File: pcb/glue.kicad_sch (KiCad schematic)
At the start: 63 parts, among them SW1 Opts, SW2 Reset Vector, SW3 NMI, SW4 RESET, U10 GAL16V8, U12 MCP100-475D, U2 74LS573, U3 74LS573, U4 74LS245, U5 74LS245, U6 74AHC273, U7 74LS240, U8 74LS240, U9 74LS259

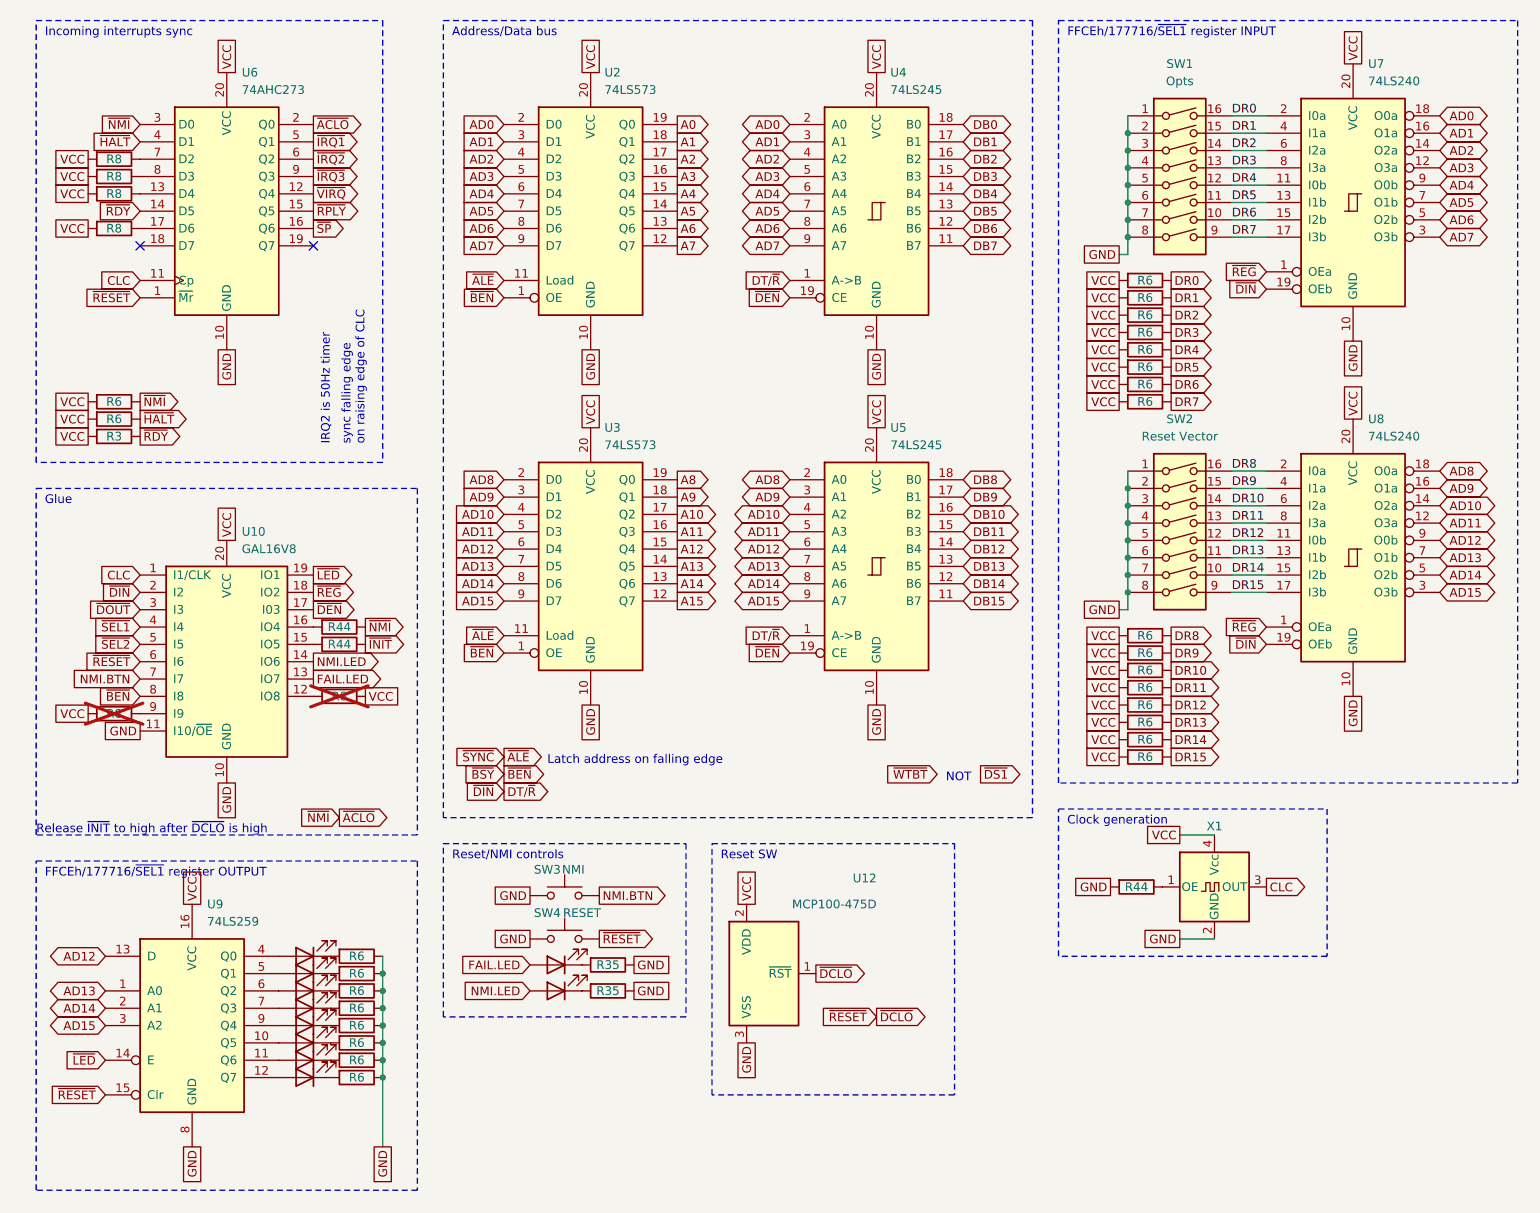
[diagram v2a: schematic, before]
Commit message: full? schematics
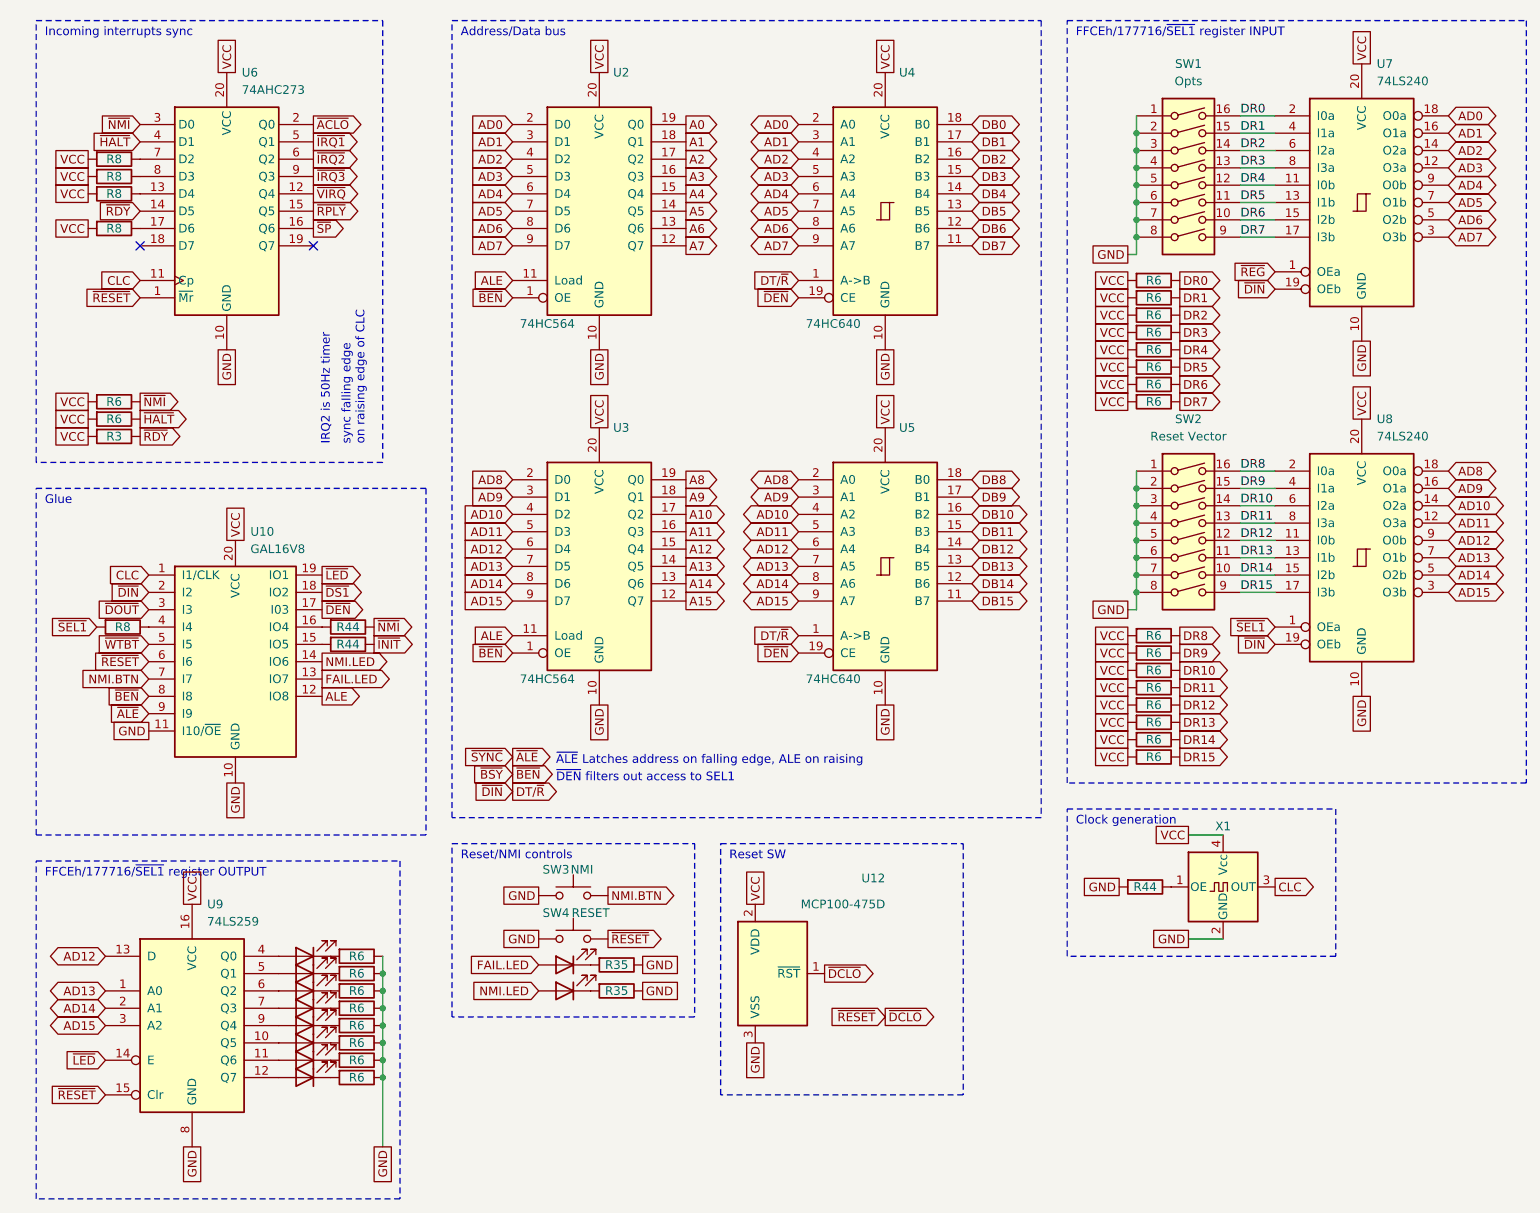
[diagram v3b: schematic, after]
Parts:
- removed R8 (x2): 0R, Resistor_SMD:R_0603_1608Metric_Pad0.98x0.95mm_HandSolder, symbol Device:R
- added R8: 0R, Resistor_SMD:R_0603_1608Metric_Pad0.98x0.95mm_HandSolder, symbol Device:R
- SW3, SW4: footprint (none) -> Button_Switch_THT:SW_SPST_Omron_B3F-315x_Angled
- U12: footprint (none) -> Package_TO_SOT_SMD:SOT-23-3
- U2, U3: value 74LS573 -> 74HC564; symbol 74xx:74LS573 -> 74xx_EXTRA:74LS564; Manufacturer_Part_Number 74VHCT573AFT -> (none); RS Part Number 171-3540 -> (none)
- U4, U5: value 74LS245 -> 74HC640; symbol 74xx:74LS245 -> 74xx_EXTRA:74LS640; Manufacturer_Name Texas Instruments -> (none); Manufacturer_Part_Number MC74HCT245ADWG -> (none); Mouser Part Number 863-MC74HCT245ADWG -> (none)
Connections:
- net ~{SEL2} is gone; now on net ~{WTBT}: U10.5 (I5)
- net ~{ACLO}: no longer R44.1, R6.1, U6.3 (D0)
- net ~{ALE}: now also U10.9 (I9); no longer U2.11 (Load), U3.11 (Load)
- net ~{DS1}: now also U10.18 (IO2)
- net ~{REG}: no longer U10.18 (IO2), U8.1 (OEa)
- net ~{SEL1}: now also U8.1 (OEa), R8.2; no longer U10.4 (I4)
- net ALE: now reaches U10.12 (IO8)
- net ALE: now also U2.11 (Load), U3.11 (Load)
- new net: R8.1, U10.4 (I4)
- new net ~{NMI}: R44.1, R6.1, U6.3 (D0)
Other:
- note added: "~{ALE} Latches address on falling edge, ALE on raising"
- note added: "~{DEN} filters out access to SEL1"
- note removed: "Latch address on falling edge"
- note removed: "NOT"
- note removed: "Release ~{INIT} to high after ~{DCLO} is high"
- moved on the sheet: R35, R44, R6, SW1, SW2, SW3, SW4, U10, U12, U2, U3, U4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

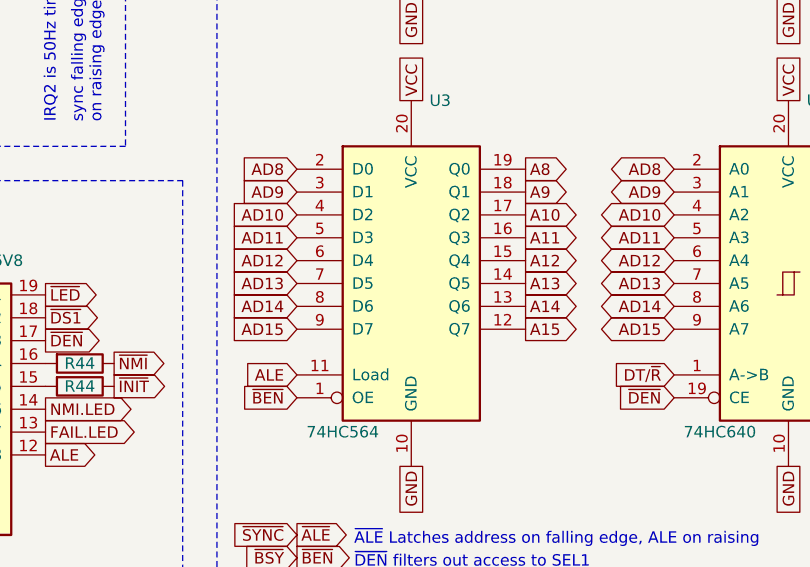
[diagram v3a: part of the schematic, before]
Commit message: placement/routing
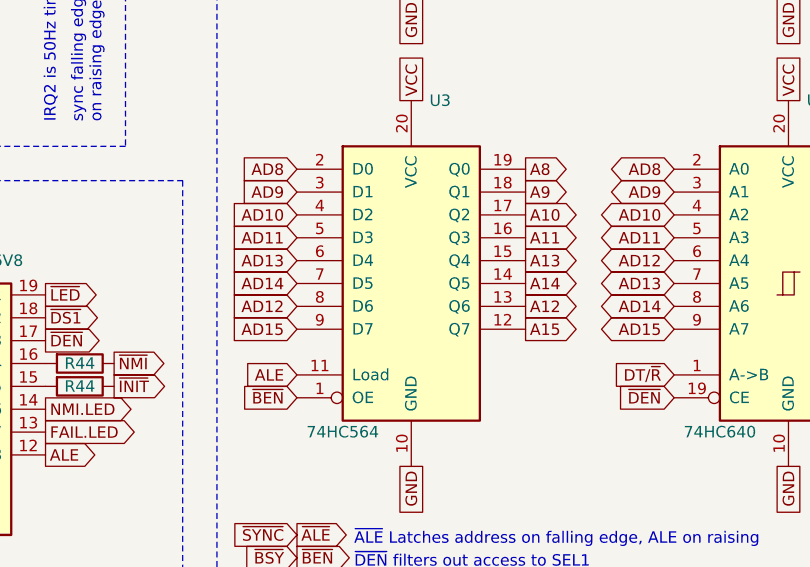
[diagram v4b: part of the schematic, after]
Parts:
- R44: value 0R -> WEAKR
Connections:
- net A12: now also U3.13 (Q6); no longer U3.15 (Q4)
- net A13: now also U3.15 (Q4); no longer U3.14 (Q5)
- net A14: now also U3.14 (Q5); no longer U3.13 (Q6)
- net AD12: now also U3.8 (D6); no longer U3.6 (D4)
- net AD13: now also U3.6 (D4); no longer U3.7 (D5)
- net AD14: now also U3.7 (D5); no longer U3.8 (D6)
